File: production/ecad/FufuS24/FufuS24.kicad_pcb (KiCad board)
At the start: 4 copper layers, 120 x 120 mm, 146 parts, among them IC1 NLVPCA9535EDTR2G, J1 Conn_01x02, J10 691137710002, J12 691137710002, J13 5033950410, J2 Conn_01x02, J3 HDMI_A, J4 USB_B_Micro, J5 691137710004, J6 5025840270, J7 691137710002, J8 691137710004, J9 5025840270, Q1 DMG2302UK-7, U1 RP2040, U10 TPD4E1U06DBVR, U11 TPD4E1U06DBVR, U12 Pololu_DRV8711_Motor_Driver, U2 W25Q128JVS, U3 TPD2E001DRLR, U4 TPS785, U5 PLMR38020FDDAR, U6 PLMR38020FDDAR, U7 PLMR38020FDDAR

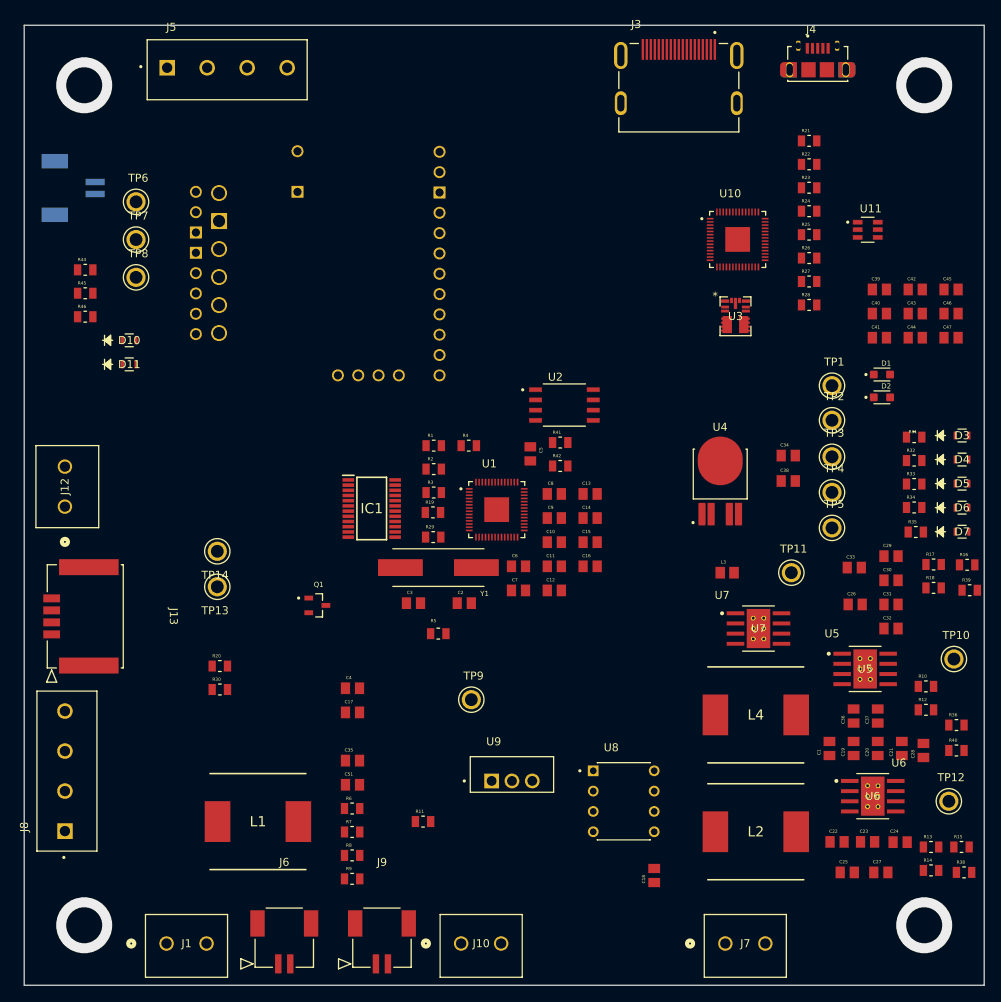
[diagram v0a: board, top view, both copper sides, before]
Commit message: efan part 2 laying out
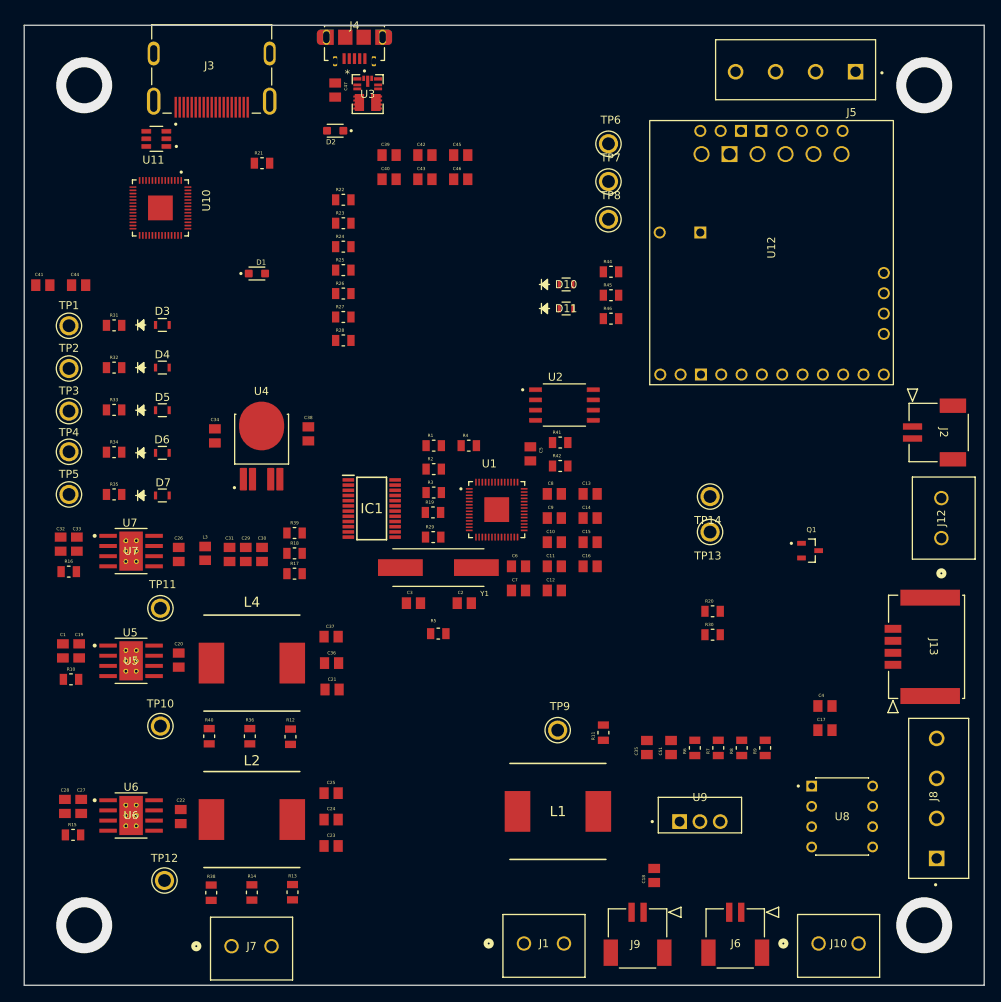
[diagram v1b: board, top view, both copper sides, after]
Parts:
- J2, U12: moved to F.Cu
- moved R16 112.3 mm to (85.6, 98.3)
- moved R15 111.1 mm to (86.1, 131.2), turned to 180 degrees
- moved J12 109.6 mm to (194.6, 94.1)
- moved J8 109.0 mm to (194.1, 134.1)
- moved C28 107.5 mm to (85.1, 127.6)
- moved R10 106.9 mm to (85.9, 111.8)
- moved J2 106.6 mm to (191.0, 80.2)
- moved J13 105.2 mm to (188.6, 109.9)
- moved C41 104.8 mm to (82.3, 62.5)
- moved C44 104.8 mm to (86.8, 62.5)
- moved C32 104.3 mm to (84.6, 94.9), turned to 90 degrees
- moved R31 101.0 mm to (91.2, 67.5)
- moved D3 100.9 mm to (97.3, 67.5)
- moved R32 100.7 mm to (91.2, 72.8)
- moved D4 100.6 mm to (97.3, 72.8)
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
